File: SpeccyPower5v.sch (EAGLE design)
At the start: 63 parts, among them T1 TRANS_ER29

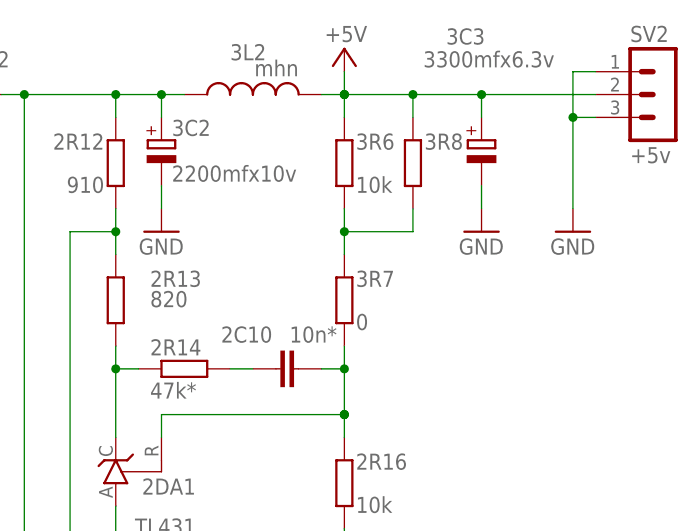
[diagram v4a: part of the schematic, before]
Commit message: ..
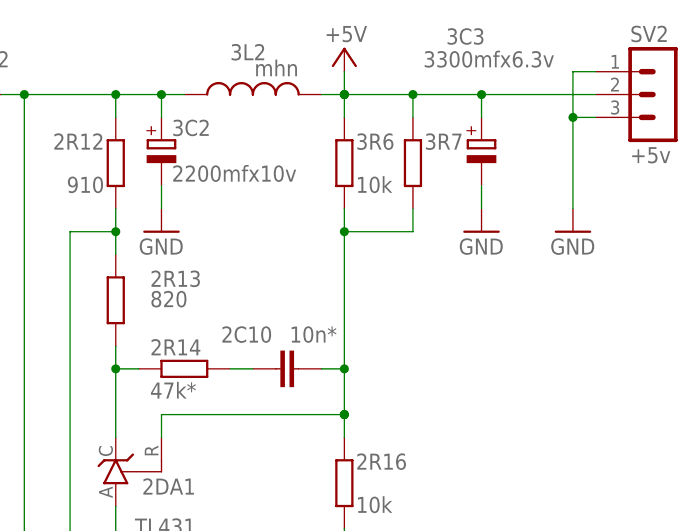
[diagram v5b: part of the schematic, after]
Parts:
- removed 3R8: (no value), rcl:R-EU_R0805
- 3C3: device SpeccyPower5v:CPOL-EUTT2D7L -> SpeccyPower5v:CPOL-EUTT2D7L-2
- 3R7: value 0 -> (none); device rcl:R-EU_M0805 -> rcl:R-EU_R0805
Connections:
- removed net N$42: 2C10.1, 2DA1.R, 2R16.2, 3R7.1
- net +5V: now also 3R7.2; no longer 3R8.2
- net N$26: now also 2C10.1, 2DA1.R, 2R16.2, 3R7.1; no longer 3R7.2, 3R8.1
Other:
- moved on the sheet: 3R7

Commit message: ..
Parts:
- 2R9: device rcl:R-EU_0207/10 -> rcl:R-EU_0204/7
- 2VD2: device SpeccyPower5v:1N4148DO35-7 -> SpeccyPower5v:1N4148DO35-10
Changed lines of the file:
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@@
 <part name="2R5" library="rcl" deviceset="R-EU_" device="0207/10" value="10k"/>
 <part name="2C3" library="rcl" deviceset="CPOL-EU" device="E2.5-6" value="100x25v"/>
-<part name="2R9" library="rcl" deviceset="R-EU_" device="0207/10" value="100"/>
+<part name="2R9" library="rcl" deviceset="R-EU_" device="0204/7" value="100"/>
 <part name="2VD3" library="SpeccyPower5v" deviceset="1N4148" device="DO35-7" value="1N4148"/>
 <part name="2R12" library="rcl" deviceset="R-EU_" device="R0805" value="910"/>
@@
 <part name="1F1" library="fuse" deviceset="SHK20L" device=""/>
 <part name="GND5" library="supply1" deviceset="GND" device=""/>
-<part name="2VD2" library="SpeccyPower5v" deviceset="1N4148" device="DO35-7" value="FR207"/>
+<part name="2VD2" library="SpeccyPower5v" deviceset="1N4148" device="DO35-10" value="FR207"/>
 <part name="1VD1" library="diode" deviceset="1N4004" device="" value="1N4007"/>
 <part name="1VD2" library="diode" deviceset="1N4004" device="" value="1N4007"/>
